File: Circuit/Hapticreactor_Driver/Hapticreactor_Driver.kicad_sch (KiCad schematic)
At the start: 3 parts

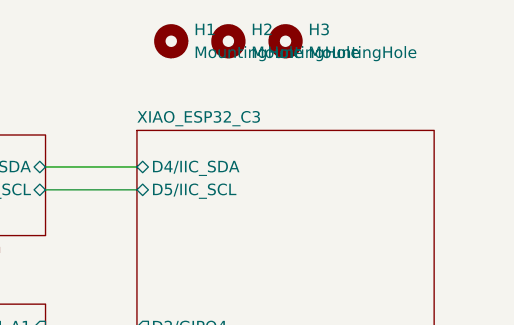
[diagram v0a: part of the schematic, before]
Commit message: ハプティックリアクタ用基板完成
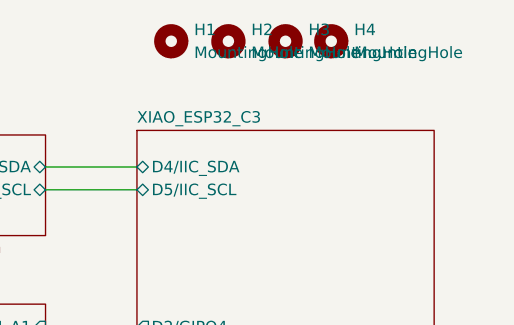
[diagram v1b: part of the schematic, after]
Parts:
- added H4: MountingHole, MountingHole:MountingHole_2.2mm_M2, symbol Mechanical:MountingHole
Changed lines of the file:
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@@
+		)
+	)
+	(symbol
+		(lib_id "Mechanical:MountingHole")
+		(at 128.27 46.99 0)
+		(unit 1)
+		(exclude_from_sim yes)
+		(in_bom no)
+		(on_board yes)
+		(dnp no)
+		(fields_autoplaced yes)
+		(property "Reference" "H4"
+			(at 130.81 45.7199 0)
+			(effects
+				(font
+					(size 1.27 1.27)
+				)
+				(justify left)
+			)
+		)
+		(property "Value" "MountingHole"
+			(at 130.81 48.2599 0)
+			(effects
+				(font
+					(size 1.27 1.27)
+				)
+				(justify left)
+			)
+		)
+		(property "Footprint" "MountingHole:MountingHole_2.2mm_M2"
+			(at 128.27 46.99 0)
+			(effects
+				(font
+					(size 1.27 1.27)
+				)
+				(hide yes)
+			)
+		)
+		(property "Datasheet" "~"
+			(at 128.27 46.99 0)
+			(effects
+				(font
+					(size 1.27 1.27)
+				)
+				(hide yes)
+			)
+		)
+		(property "Description" "Mounting Hole without connection"
+			(at 128.27 46.99 0)
+			(effects
+				(font
+					(size 1.27 1.27)
+				)
+				(hide yes)
+			)
+		)
+		(instances
+			(project "Hapticreactor_Driver"
+				(path "/2de60640-83cc-436b-97a4-426b15b610d6"
+					(reference "H4")
+					(unit 1)
+				)
+			)
 		)
 	)
